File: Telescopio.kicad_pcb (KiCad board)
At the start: 2 copper layers, 201.9 x 119.4 mm, 19 parts, among them CON1 BARREL_JACK, P1 CONN_01X03, P10 CONN_01X08, P12 CONN_01X04, P13 CONN_01X04, P2 CONN_01X03, P3 CONN_01X05, P4 CONN_01X19, P5 CONN_01X19, P50 CONN_01X04, P51 CONN_01X10, P7 CONN_01X08, P8 CONN_01X08, P9 CONN_01X08, SW1 SW_PUSH

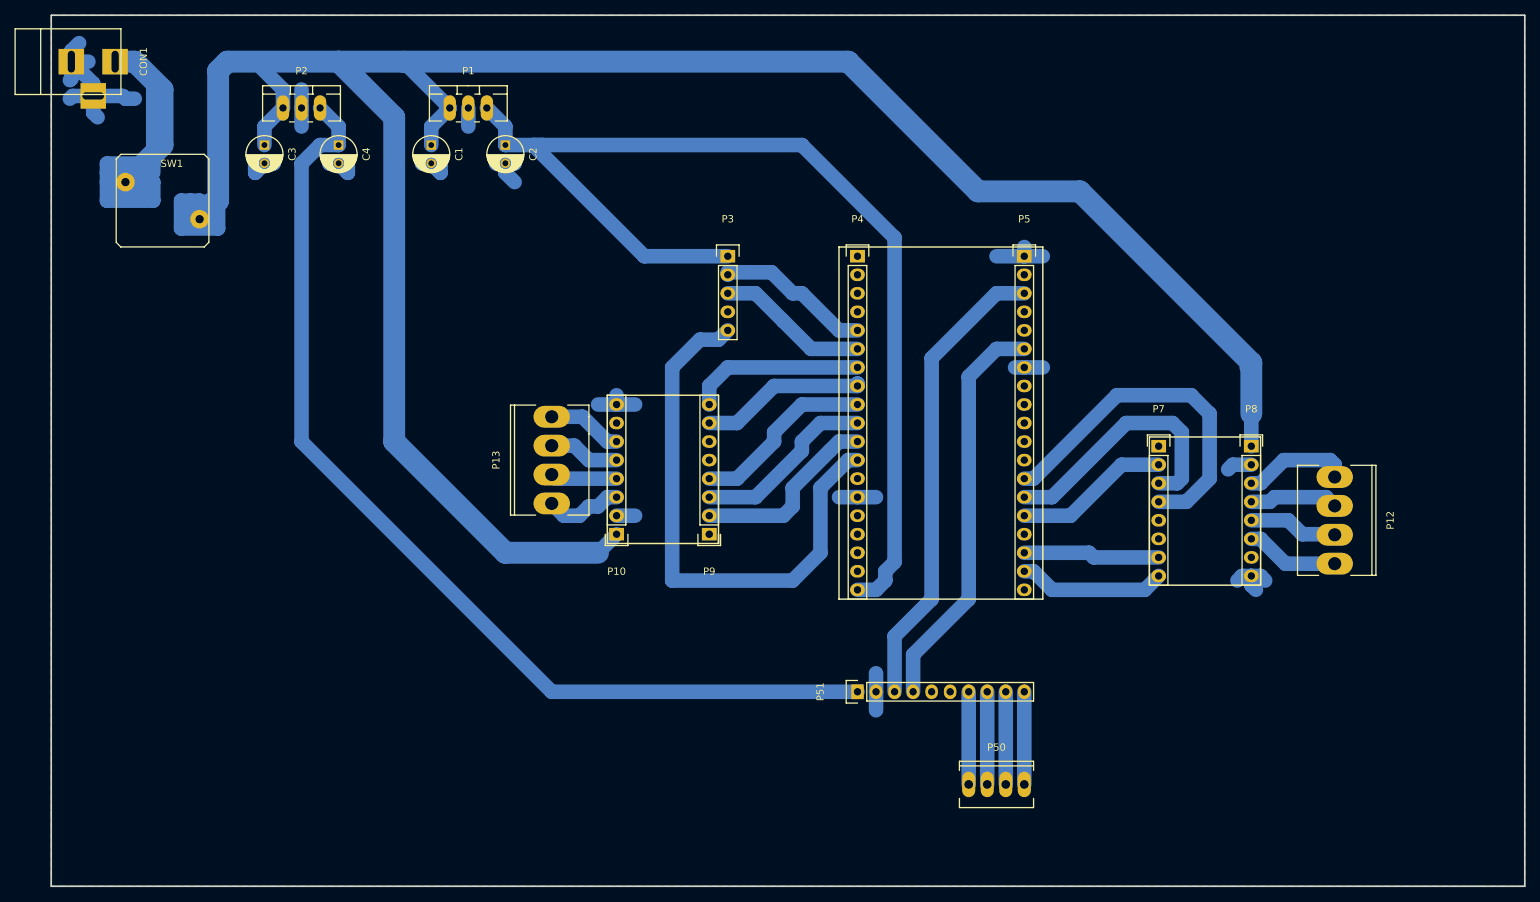
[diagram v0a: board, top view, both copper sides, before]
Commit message: modifed pcb for testing
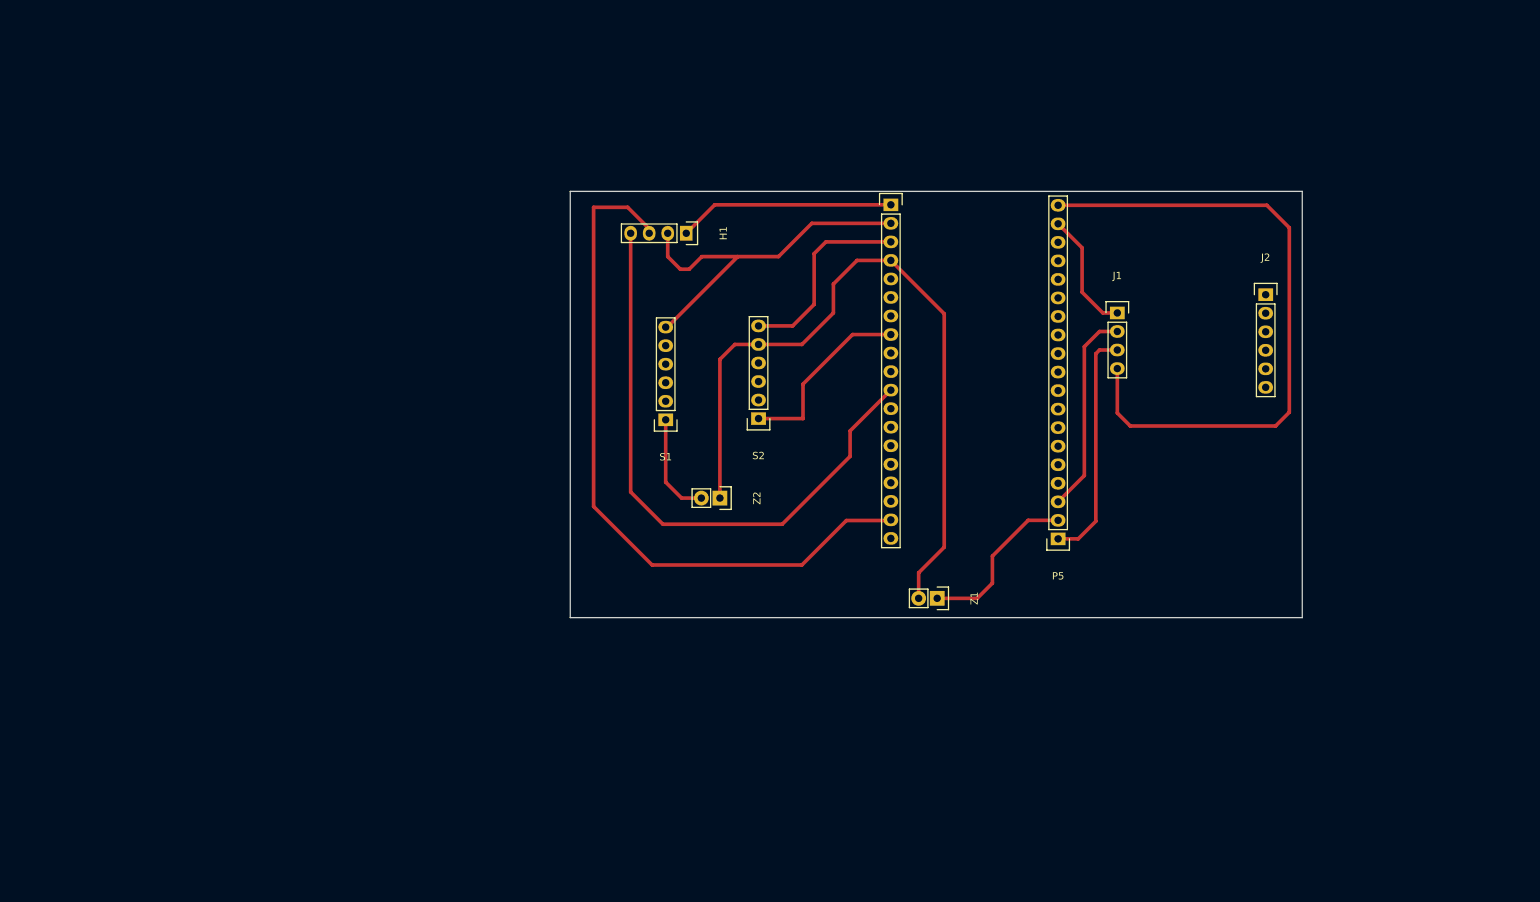
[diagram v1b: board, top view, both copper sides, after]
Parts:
- removed C1, C2, C3, C4: C, Capacitors_ThroughHole:C_Radial_D5_L11_P2.5
- removed CON1: BARREL_JACK, Connect:BARREL_JACK
- removed P1, P2: CONN_01X03, TO_SOT_Packages_THT:TO-220_Neutral123_Vertical_LargePads
- removed P10, P7, P8, P9: CONN_01X08, Pin_Headers:Pin_Header_Straight_1x08
- removed P12, P13: CONN_01X04, Sockets_MOLEX_KK-System:Socket_MOLEX-KK-RM3-96mm_Lock_4pin_straight
- removed P3: CONN_01X05, Pin_Headers:Pin_Header_Straight_1x05
- removed P50: CONN_01X04, Sockets_MOLEX_KK-System:Socket_MOLEX-KK-RM2-54mm_Lock_4pin_straight
- removed P51: CONN_01X10, Pin_Headers:Pin_Header_Straight_1x10
- removed SW1: SW_PUSH, Buttons_Switches_ThroughHole:SW_PUSH
- added H1: Temp_humidity, Pin_Headers:Pin_Header_Straight_1x04, F.Cu at (107.3, 57.8)
- added J1: ScaleL, Pin_Headers:Pin_Header_Straight_1x04, F.Cu at (166.4, 68.7)
- added J2: Scale, Pin_Headers:Pin_Header_Straight_1x06, F.Cu at (186.8, 66.2)
- added S1: Shifter, Pin_Headers:Pin_Header_Straight_1x06, F.Cu at (104.5, 83.4)
- added S2: ShifterR, Pin_Headers:Pin_Header_Straight_1x06, F.Cu at (117.2, 83.2)
- added Z1: Buzzer, Pin_Headers:Pin_Header_Straight_1x02, F.Cu at (141.7, 107.8)
- added Z2: Motor, Pin_Headers:Pin_Header_Straight_1x02, F.Cu at (112.0, 94.1)
- P4: value CONN_01X19 -> ESP_32
- P5: value CONN_01X19 -> esp_lora
- moved P5 39.0 mm to (158.3, 99.7), turned to 180 degrees
- moved P4 8.40 mm to (135.4, 53.9)
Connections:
- P4 pad 1: (no net) -> /GND2
- P4 pad 10: /M1_2 -> Net-(P4-Pad10)
- P4 pad 11: /M0_2 -> /SCL
- P4 pad 12: /INT_IMU -> Net-(P4-Pad12)
- P4 pad 13: (no net) -> Net-(P4-Pad13)
- P4 pad 14: GND -> Net-(P4-Pad14)
- P4 pad 15: (no net) -> Net-(P4-Pad15)
- P4 pad 16: (no net) -> Net-(P4-Pad16)
- P4 pad 17: (no net) -> Net-(P4-Pad17)
- P4 pad 18: (no net) -> /SDA
- P4 pad 19: /5v -> Net-(P4-Pad19)
- P4 pad 2: (no net) -> /5v1
- P4 pad 3: (no net) -> /3v
- P4 pad 4: (no net) -> /GND
- P4 pad 5: /SCL_2 -> Net-(P4-Pad5)
- P4 pad 6: /SDA_2 -> Net-(P4-Pad6)
- P4 pad 7: /Dir_2 -> Net-(P4-Pad7)
- P4 pad 8: /Step_2 -> /M0
- P4 pad 9: /M2_2 -> Net-(P4-Pad9)
- P5 pad 1: GND -> /DT
- P5 pad 10: (no net) -> Net-(P5-Pad10)
- P5 pad 11: (no net) -> Net-(P5-Pad11)
- P5 pad 12: (no net) -> Net-(P5-Pad12)
- P5 pad 13: /M2_1 -> Net-(P5-Pad13)
- P5 pad 14: /M1_1 -> Net-(P5-Pad14)
- P5 pad 15: /M0_1 -> Net-(P5-Pad15)
- P5 pad 16: (no net) -> Net-(P5-Pad16)
- P5 pad 17: /Step_1 -> Net-(P5-Pad17)
- P5 pad 18: /Dir_1 -> /VCC
- P5 pad 19: (no net) -> /GND1
- P5 pad 2: (no net) -> Net-(P5-Pad2)
- P5 pad 3: /SCL -> /SCK
- P5 pad 4: (no net) -> Net-(P5-Pad4)
- P5 pad 5: (no net) -> Net-(P5-Pad5)
- P5 pad 6: /SDA -> Net-(P5-Pad6)
- P5 pad 7: GND -> Net-(P5-Pad7)
- P5 pad 8: (no net) -> Net-(P5-Pad8)
- P5 pad 9: (no net) -> Net-(P5-Pad9)
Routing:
- net /24v_Sal: track 373.3 -> 0.00 mm
- net /5v: track 150.8 -> 0.00 mm
- net /3v3: track 140.8 -> 0.00 mm
- net /GND: track 0.00 -> 101.2 mm
- net GND: track 97.0 -> 0.00 mm
- net /GND1: track 0.00 -> 89.4 mm
- net /24v: track 80.6 -> 0.00 mm
- net /INT_IMU: track 76.4 -> 0.00 mm
- net /5v1: track 0.00 -> 51.0 mm
- net /M2_1: track 48.4 -> 0.00 mm
- net /SDA: track 55.5 -> 97.1 mm
- net /M1_1: track 36.1 -> 0.00 mm
- net /DT: track 0.00 -> 32.3 mm
- net /GND2: track 0.00 -> 29.7 mm
- net /SCK: track 0.00 -> 28.1 mm
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- removed copper zone on B.Cu, net GND
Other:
- board size 201.9 x 119.4 mm -> 100.3 x 58.4 mm
